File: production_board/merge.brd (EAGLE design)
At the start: 100 x 100 mm, 87 parts, among them Q1 FC-12M, Q2 FC-12M, Q3 FC-12M, U1 MDBT40SMD, U2 MPU-9250, U3 MDBT40SMD, U4 MPU-9250, U5 MDBT40SMD, U6 MPU-9250

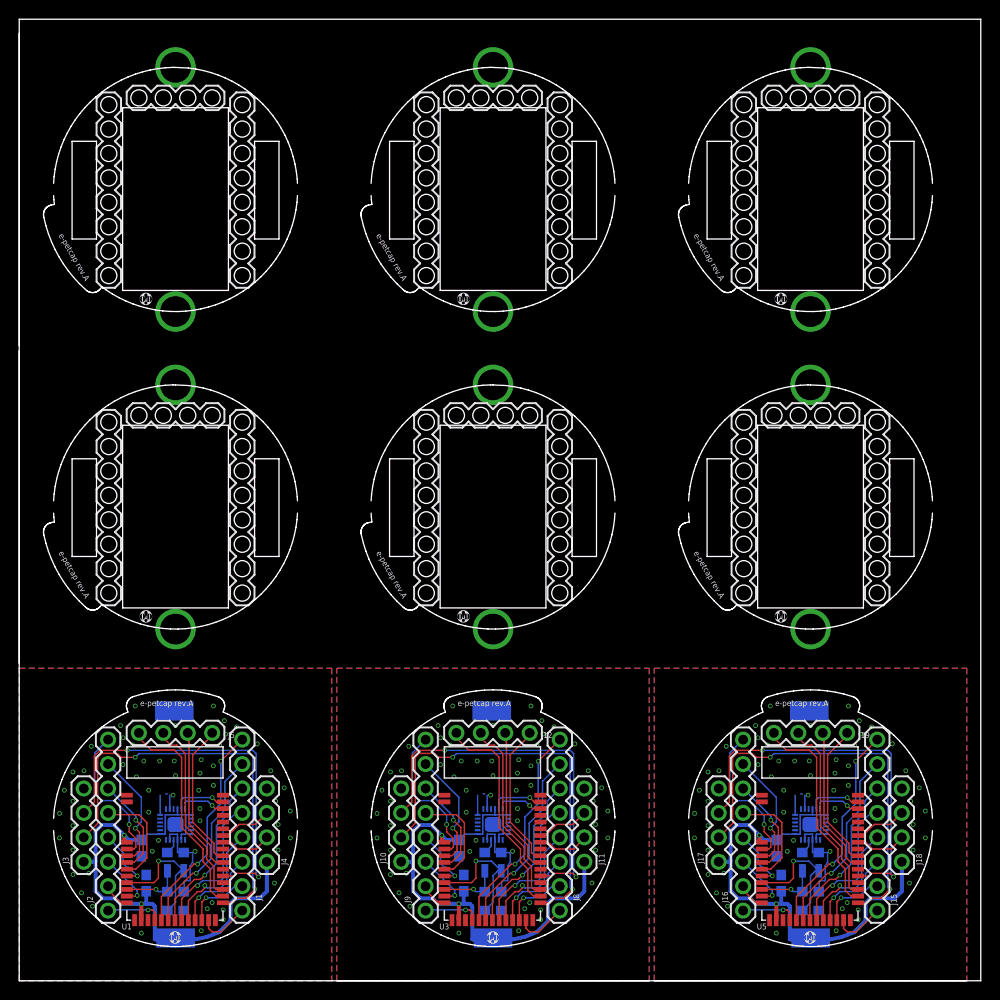
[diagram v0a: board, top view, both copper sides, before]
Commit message: before order r2 board
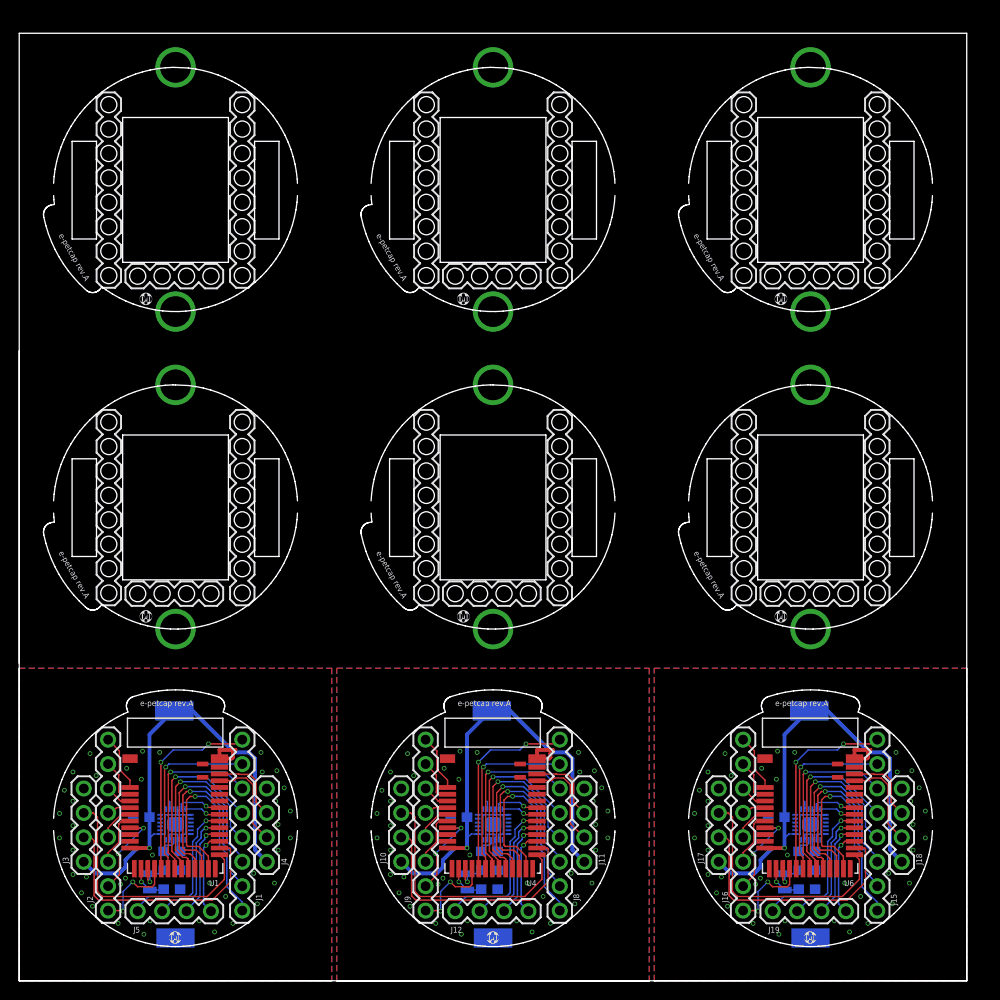
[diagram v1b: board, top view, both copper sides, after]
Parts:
- removed C13, C15: 1uF, SparkFun-Capacitors:0603-CAP
- removed C14: .1uF, SparkFun-Capacitors:0603-CAP
- C10: value 1uF -> 12pF
- C11: value 12pF -> 10uF
- C12: value 12pF -> 1uF
- C3: value 1uF -> 10uF
- C5: value .1uF -> 10uF
- C9: value .1uF -> 12pF
- U1: value MDBT40SMD -> MDBT42SMD; device MDBT40:MDBT40 -> MDBT42:MDBT42
- U3, U5: value MDBT40SMD -> MPU-9250; device MDBT40:MDBT40 -> invensense:LEAD-QFN24
- U4, U6: value MPU-9250 -> MDBT42SMD; device invensense:LEAD-QFN24 -> MDBT42:MDBT42
- moved C9 36.3 mm to (81.9, 11.5), turned to 180 degrees
- moved C5 33.2 mm to (45.7, 17.0), turned to 0 degrees
- moved C10 32.9 mm to (81.9, 9.53), turned to 180 degrees
- moved J13 23.6 mm to (49.3, 4.45)
- moved J14 23.6 mm to (49.1, 28.1)
- moved J20 23.6 mm to (82.3, 4.45)
- moved J21 23.6 mm to (82.2, 28.1)
- moved J6 23.6 mm to (16.3, 4.45)
- moved J7 23.6 mm to (16.1, 28.1)
- moved U$13 20.1 mm to (78.4, 40.3), turned to 0 degrees
- moved U$23 20.1 mm to (45.3, 73.3), turned to 0 degrees
- moved U$28 20.1 mm to (78.4, 73.3), turned to 0 degrees
- moved U$8 20.1 mm to (45.3, 40.3), turned to 0 degrees
- moved J12 20.1 mm to (45.3, 7.24), turned to 0 degrees
- moved J19 20.1 mm to (78.4, 7.24), turned to 0 degrees
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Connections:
- removed net LED4: U1.37, U3.37, U5.37
- removed net N$1: C2.1, Q2.1, U3.9
- removed net N$10: C4.1, Q2.2, U3.10
- removed net N$11: C10.2, U4.10
- removed net N$17: C11.1, Q3.1, U5.9
- removed net N$18: C12.1, Q3.2, U5.10
- removed net N$19: C15.2, U6.10
- new net LED0: U1.34, U4.34, U6.34
- new net LED1: U1.33, U4.33, U6.33
- new net N$100: C4.1, Q2.2, U4.13
- new net N$101: C8.2, U3.10
- new net N$107: C9.1, Q3.1, U6.14
- new net N$108: C10.1, Q3.2, U6.13
- new net N$109: C12.2, U5.10
- new net N$64: C2.1, Q2.1, U4.14
- new net NRESET: U1.35, U4.35, U6.35
- net A0: now also U1.16, U4.16, U6.16; no longer U1.17, U3.17, U5.17
- net A1: now also U1.17, U4.17, U6.17; no longer U1.18, U3.18, U5.18
- net A2: now also U1.18, U4.18, U6.18; no longer U1.19, U3.19, U5.19
- net A3: now also U1.19, U4.19, U6.19; no longer U1.20, U3.20, U5.20
- net A4: now also U1.20, U4.20, U6.20; no longer U1.21, U3.21, U5.21
- net A5: now also U1.21, U4.21, U6.21; no longer U1.22, U3.22, U5.22
- net A6: now also U1.22, U4.22, U6.22; no longer U1.23, U3.23, U5.23
- net A7: now also U1.23, U4.23, U6.23; no longer U1.24, U3.24, U5.24
- net D0: now also U1.2, U4.2, U6.2; no longer U1.4, U3.4, U5.4
- net D1: now also U1.3, U4.3, U6.3; no longer U1.5, U3.5, U5.5
- net D2: now also U1.4, U4.4, U6.4; no longer U1.6, U3.6, U5.6
- net D3: now also U1.5, U4.5, U6.5; no longer U1.7, U3.7, U5.7
- net D4: now also U1.6, U4.6, U6.6; no longer U1.8, U3.8, U5.8
- net D5: now also U1.7, U4.7, U6.7; no longer U1.11, U3.11, U5.11
- net D6: now also U1.8, U4.8, U6.8; no longer U1.12, U3.12, U5.12
- net D7: now also U1.15, U4.15, U6.15; no longer U1.16, U3.16, U5.16
- net GND: now also C10.2, C12.1, C8.1, U1.12, U1.24, U1.39, U3.11, U3.18, U3.20, U3.9, U4.1, U4.12, U4.24, U4.39, U5.11, U5.18, U5.20, U5.9, U6.1, U6.12, U6.24, U6.39; no longer C10.1, C12.2, C13.2, C14.2, C15.1, C8.2, U1.13, U1.2, U1.25, U1.42, U3.1, U3.13, U3.2, U3.25, U3.42, U4.11, U4.18, U4.20, U4.9, U5.1, U5.13, U5.2, U5.25, U5.42, U6.11, U6.18, U6.20, U6.9
- net N$2: now also U1.14; no longer U1.9
- net N$3: now also U1.13; no longer U1.10
- net RX: now also U1.25, U4.25, U6.25; no longer U1.30, U3.30, U5.30
- net SPI_MISO: now also U1.29, U4.29, U6.29; no longer U1.32, U3.32, U5.32
- net SPI_MOSI: now also U4.27, U6.27; no longer U3.27, U5.27
- net SPI_SCK: now also U4.28, U6.28; no longer U3.28, U5.28
- net SPI_SS: now also U1.30, U4.30, U6.30; no longer U1.33, U3.33, U5.33
- net SWCLK: now also J11.2, J18.2, J4.2, U4.36, U6.36; no longer J11.3, J18.3, J4.3, U3.36, U5.36
- net SWDIO: now also J11.3, J18.3, J4.3, U1.37, U4.37, U6.37; no longer J11.2, J18.2, J4.2, U1.35, U3.35, U5.35
- net TWI_SCL: now also U1.32, U3.23, U4.32, U5.23, U6.32; no longer U1.41, U3.41, U4.23, U5.41, U6.23
- net TWI_SDA: now also U1.31, U3.24, U4.31, U5.24, U6.31; no longer U1.40, U3.40, U4.24, U5.40, U6.24
- net TX: now also U4.26, U6.26; no longer U3.26, U5.26
- net VCC: now also C11.1, U1.11, U3.1, U3.13, U3.22, U3.8, U4.11, U5.1, U5.13, U5.22, U5.8, U6.11; no longer C13.1, C14.1, C8.1, C9.1, U1.14, U1.3, U3.14, U3.3, U4.1, U4.13, U4.22, U4.8, U5.14, U5.3, U6.1, U6.13, U6.22, U6.8
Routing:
- net A7: track 16.3 -> 73.7 mm, vias 0 -> 3
- net TX: track 130.4 -> 80.1 mm, vias 6 -> 0
- net A6: track 20.3 -> 69.5 mm
- net RX: track 121.5 -> 78.8 mm, vias 6 -> 0
- net SPI_MOSI: track 67.3 -> 27.6 mm, vias 0 -> 3
- net A5: track 27.7 -> 64.2 mm
- net SPI_SCK: track 58.9 -> 30.5 mm, vias 0 -> 3
- net D0: track 45.9 -> 17.8 mm, vias 3 -> 0
- net D3: track 32.0 -> 7.53 mm
- net D6: track 8.73 -> 32.9 mm, vias 0 -> 6
- net D1: track 37.3 -> 13.9 mm, vias 3 -> 0
- net A4: track 37.5 -> 60.6 mm
- net D2: track 31.1 -> 8.46 mm, vias 3 -> 0
- net SWCLK: track 16.6 -> 29.9 mm
- net N$17: track 13.3 -> 0.00 mm, vias 1 -> 0
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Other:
- board size 100 x 100 mm -> 98.5 x 98.5 mm
